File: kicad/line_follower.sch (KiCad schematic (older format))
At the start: 43 parts, among them J1 XT30PW-M, M1 MOTOR_ENC, M2 MOTOR_ENC, Q1 ALS-PT19-315C_L177_TR8, Q2 ALS-PT19-315C_L177_TR8, Q3 ALS-PT19-315C_L177_TR8, Q4 ALS-PT19-315C_L177_TR8, Q5 ALS-PT19-315C_L177_TR8, SW1 SW_Push, U1 A4950E, U2 A4950E, U3 NCV4274CDT50RKG, X1 ESP32_DEVKITV1, X2 GY-521-module, X3 DISTANCE_SENSOR

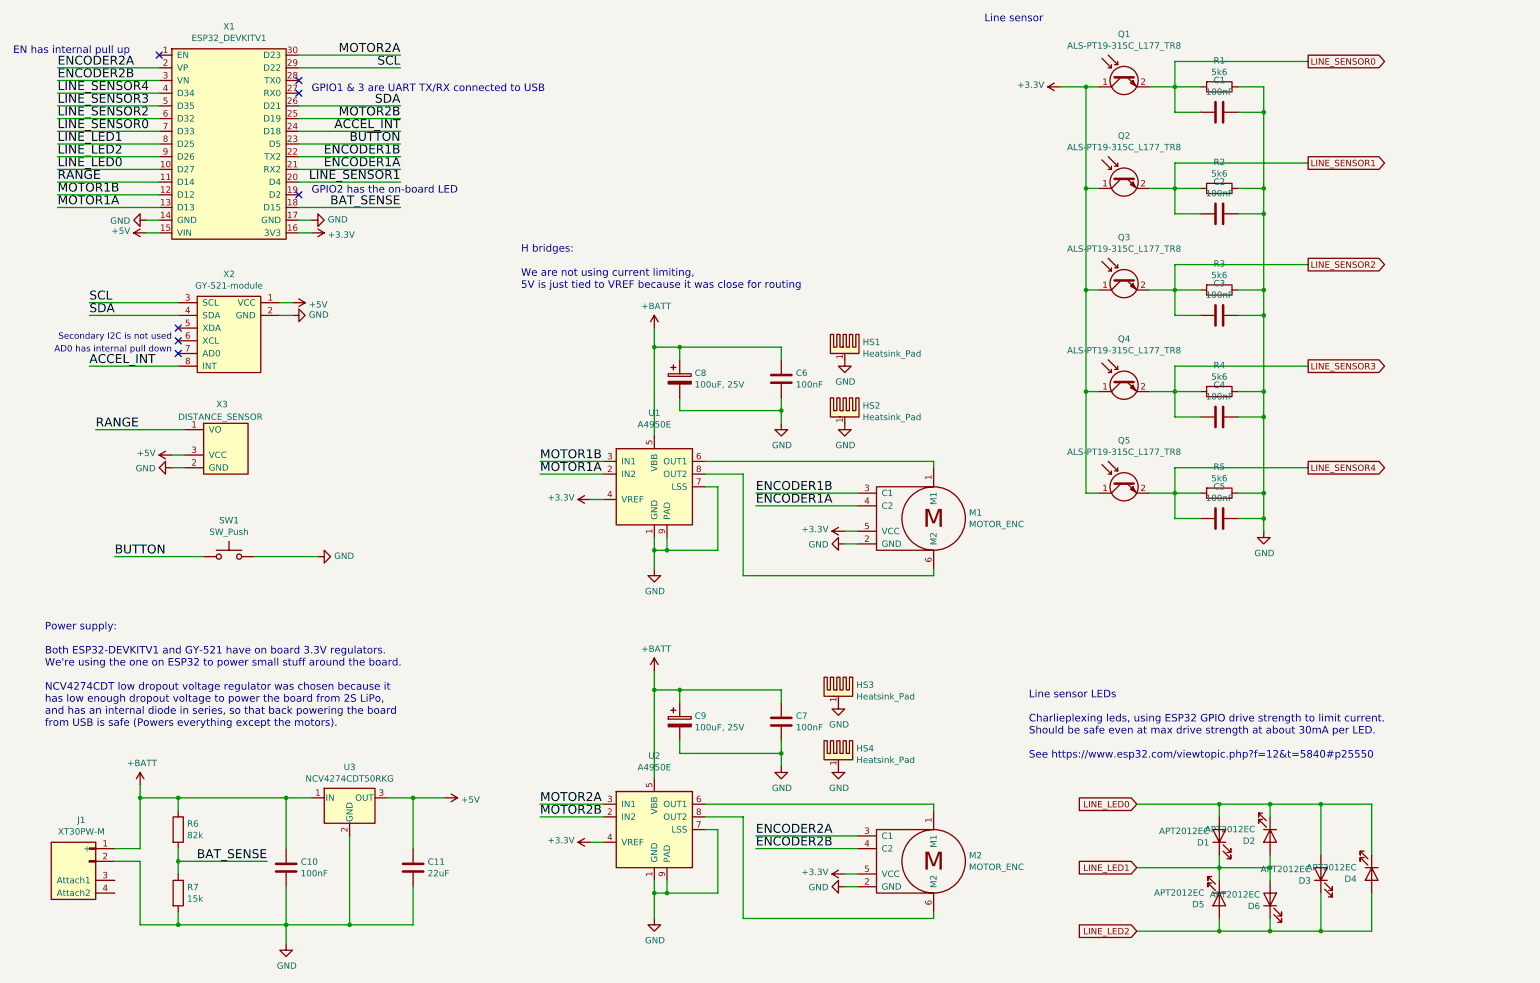
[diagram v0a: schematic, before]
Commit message: Board done except for the motor mounts
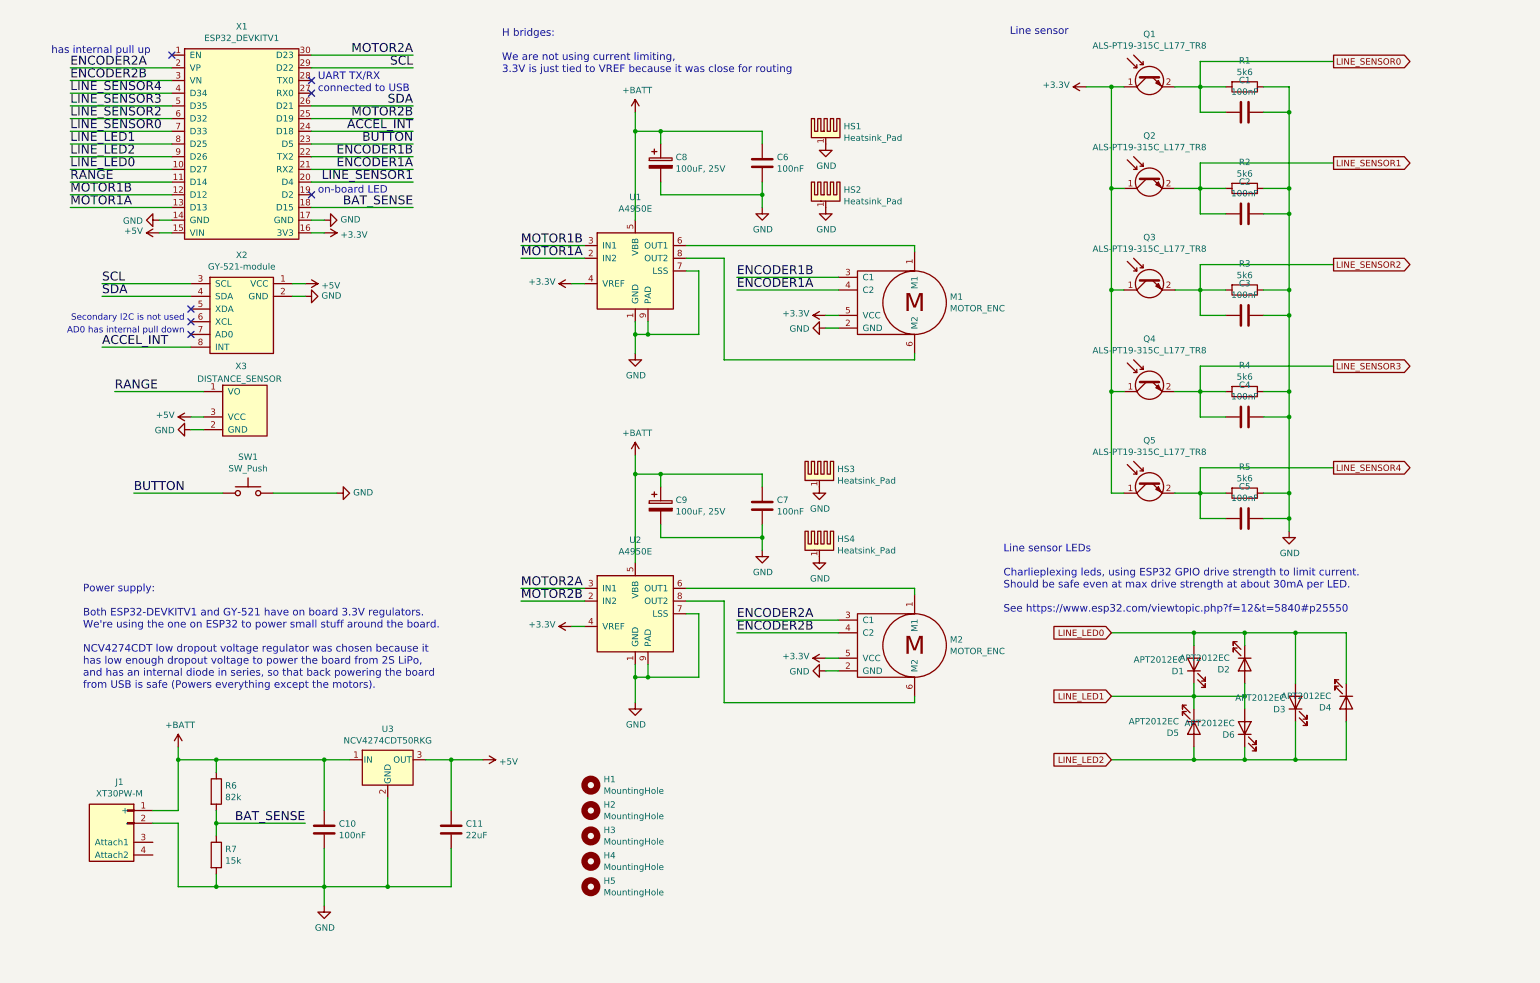
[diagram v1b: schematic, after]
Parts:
- added H1, H2, H3, H4, H5: MountingHole, MountingHole:MountingHole_3.2mm_M3, symbol Mechanical:MountingHole
- M1, M2: footprint cube-library:SolderWirePad1x6_p2.54 -> cube-library:SolderWirePad2x3_p2.54_staggered
- renumbered HS4 to HS2, HS2 to HS4
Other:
- note added: "H bridges:\n\nWe are not using current limiting,\n3.3V is just tied to VREF because it was close for routing"
- note added: "UART TX/RX\nconnected to USB"
- note added: "has internal pull up"
- note added: "on-board LED"
- note removed: "EN has internal pull up"
- note removed: "GPIO1 & 3 are UART TX/RX connected to USB"
- note removed: "GPIO2 has the on-board LED"
- note removed: "H bridges:\n\nWe are not using current limiting,\n5V is just tied to VREF because it was close for routing"
- moved on the sheet: C1, C10, C11, C2, C3, C4, C5, C6, C7, C8, C9, D1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
